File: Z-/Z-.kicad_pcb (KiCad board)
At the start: 4 copper layers, 98 x 98 mm, 138 parts, among them J1 200528-0100, J2 Conn_Coaxial, J3 Conn_Coaxial, J4 200528-0100, J5 Conn_01x02, K1 IM02DGR, Q1 NX3008NBKS, Q10 NX3008NBKS, Q11 IRLML2803, Q12 MBT2222ADW1T1, Q13 IRLML2803, Q14 NX3008NBKS, Q15 IRF7404, Q16 MBT2222ADW1T1, Q17 IRF7404, Q18 IRLML2803, Q19 IRF7404, Q2 NX3008NBKS, Q3 MBT2222ADW1T1, Q4 MBT2222ADW1T1, Q5 NX3008NBKS, Q6 NX3008NBKS, Q7 MBT2222ADW1T1, Q8 MBT2222ADW1T1, Q9 MMBT2222AT, U1 OPT4003DNPRQ1, U2 LTC4316xDD, U3 ADM1176-1ARMZ-R7, U4 NCV891330PD50R2G, U5 DRV8830DRC

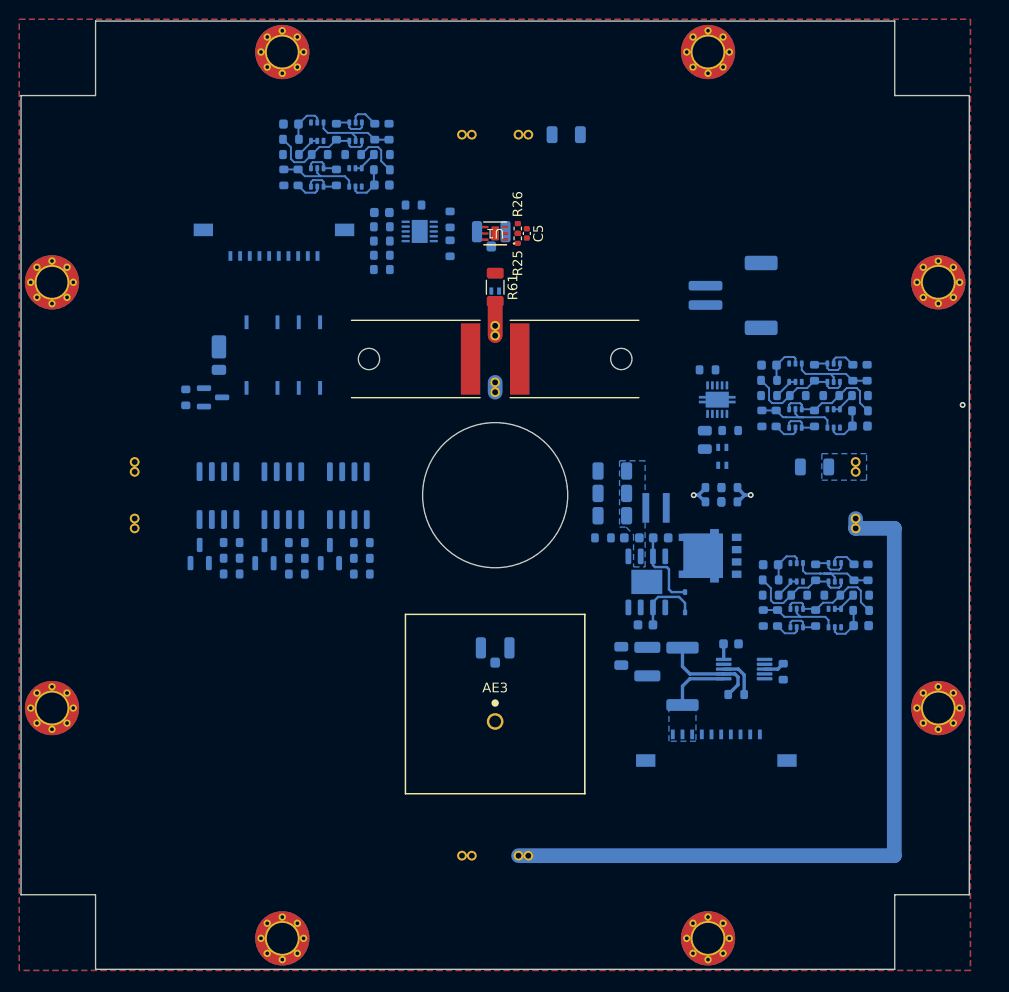
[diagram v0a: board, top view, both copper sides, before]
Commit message: Z- Board Files
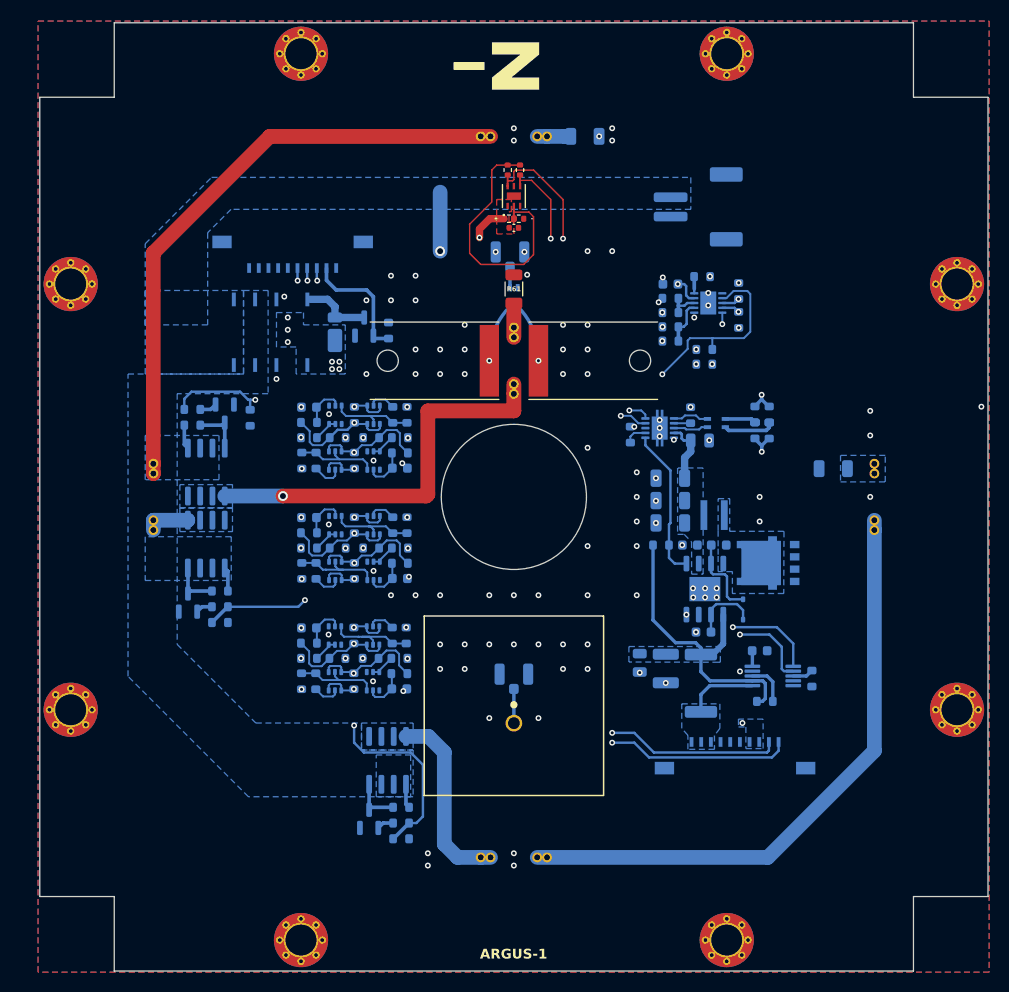
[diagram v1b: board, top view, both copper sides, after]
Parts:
- added G***: LOGO, LOGO, B.Cu at (148.1, 78.4)
- added R69: 0R (DNI), Resistor_SMD:R_0603_1608Metric, B.Cu at (169.5, 85.3)
- added R70: 0R (DNI), Resistor_SMD:R_0603_1608Metric, B.Cu at (169.5, 83.8)
- added R71: 0R, Resistor_SMD:R_0402_1005Metric, F.Cu at (149.2, 65.3)
- added R72: 0R, Resistor_SMD:R_0402_1005Metric, F.Cu at (150.5, 65.3)
- added Ref**: Val**, custom-footprints:ypanel, F.Cu at (149.4, 54.3)
- AE3: value GPS Antenna -> CGGBP.18.4.A.02
- BA1: value ATB2012-50011-T000 -> DXW21HN5011BL
- J2, J3: value Conn_Coaxial -> U.FL
- moved C2 50.1 mm to (138.1, 107.5)
- moved C4 50.1 mm to (128.7, 101.2)
- moved Q4 50.1 mm to (131.4, 106.7)
- moved Q6 50.1 mm to (131.4, 102.0)
- moved R14 50.1 mm to (138.1, 104.3)
- moved R21 50.1 mm to (135.1, 104.3)
- moved R22 50.1 mm to (138.1, 105.9)
- moved R24 50.1 mm to (137.3, 102.0)
- moved R28 50.1 mm to (128.7, 104.3)
- moved R3 50.1 mm to (129.4, 106.7)
- moved R30 50.1 mm to (138.8, 102.0)
- moved R33 50.1 mm to (131.7, 104.3)
- moved R34 50.1 mm to (128.7, 102.8)
- moved R18 50.1 mm to (127.9, 106.7)
- moved Q2 50.1 mm to (135.4, 106.7)
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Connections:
- net Net-(D2-K) renamed /I2C Devices/SW
- net Net-(U1-ADDR) renamed /I2C Devices/ADDR
- J1 pad 10: VBATT -> VBATT_SENSE
- J1 pad 8: VBATT -> VBATT_SENSE
- J1 pad 9: VBATT -> VBATT_SENSE
- J4 pad 2: BURN_RELAY_A -> GND
- J4 pad 3: BURN_EN1 -> GND
- J4 pad 4: BURN_EN2 -> GND
- J4 pad 5: BURN_EN3 -> BURN_EN4
- J4 pad 6: BURN_EN4 -> BURN_EN3
- J4 pad 7: GND -> BURN_EN2
- J4 pad 8: GND -> BURN_EN1
- J4 pad 9: GND -> BURN_RELAY_A
- J5 pad MP: (no net) -> GND
- R2 pad 2: VBATT -> VBATT_SENSE
- U3 pad 1: VBATT -> VBATT_SENSE
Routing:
- net 3.3V: track 0.00 -> 113.9 mm, vias 0 -> 26
- net SDA: track 11.4 -> 97.2 mm, vias 0 -> 4
- net SCL: track 11.5 -> 90.8 mm, vias 0 -> 4
- net BURN_EN2: track 0.00 -> 71.3 mm, vias 0 -> 2
- net Net-(JP1-Pad2): track 0.00 -> 62.6 mm
- net SDA_LS: track 8.67 -> 65.6 mm, vias 0 -> 2
- net SDA_CPWR: track 11.9 -> 63.7 mm, vias 0 -> 2
- net SCL_CPWR: track 11.9 -> 62.9 mm, vias 0 -> 2
- net SCL_LS: track 11.9 -> 61.5 mm, vias 0 -> 3
- net SCL_M: track 11.9 -> 60.6 mm, vias 0 -> 2
- net SDA_M: track 11.9 -> 60.3 mm, vias 0 -> 2
- net /I2C Devices/SDAOUT: track 0.00 -> 47.4 mm, vias 0 -> 3
- net BURN_EN1: track 0.00 -> 45.4 mm, vias 0 -> 2
- net /I2C Devices/SCLOUT: track 0.00 -> 43.0 mm, vias 0 -> 3
- net /Burn Wires/VBURN3: track 1.02 -> 41.4 mm, vias 0 -> 1
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- added copper zone on B.Cu, net /Burn Wires/VBURN1
- added copper zone on B.Cu, net /Burn Wires/VBURN2
- added copper zone on B.Cu, net /Burn Wires/VBURN3
- added copper zone on B.Cu, net /Burn Wires/VBURN_A_IN
- added copper zone on B.Cu, net /I2C Devices/SW
- added copper zone on B.Cu, net 3.3V
- added copper zone on F.Cu, net 3.3V
- added copper zone on In1.Cu, net 3.3V
- added copper zone on In1.Cu, net GND
- added copper zone on In1.Cu, net VBATT
- added copper zone on B.Cu, net VBATT_SENSE
- added copper zone on B.Cu, net VDRIVE
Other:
- board text added: "+"
- board text added: "-"
- board text added: "3.3V"
- board text added: "ALUN"
- board text added: "ARGUS-1"
- board text added: "ARGUS-1 Cubesat Carnegie Mellon University Z- Solar Panel v1"
- board text added: "BURN WIRE 1"
- board text added: "BURN WIRE 2"
- board text added: "BURN WIRE 3"
- board text added: "BURNWIRE 1"
- board text added: "BURNWIRE 2"
- board text added: "BURNWIRE 3"
- board text added: "BURN_EN1"
- board text added: "BURN_EN2"
- board text added: "BURN_EN3"
- board text added: "BURN_EN4"
- board text added: "COIL DRIVER"
- board text added: "COIL PWR MONITOR"
- board text added: "GND"
- board text added: "GPS ANT"
- board text added: "I2C ADDR TRANSLATOR"
- board text added: "I2C BUS PROTECTION"
- board text added: "MAINBOARD"
- board text added: "POWER RELAY A"
- board text added: "REGULATOR BUCK 5V"
- board text added: "RELAY_A"
- board text added: "SCL"
- board text added: "SDA"
- board text added: "UHF ANT"
- board text added: "VBATT"
